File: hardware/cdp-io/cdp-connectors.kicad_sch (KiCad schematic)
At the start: 1 part, among them J1 Conn_01x26_Pin

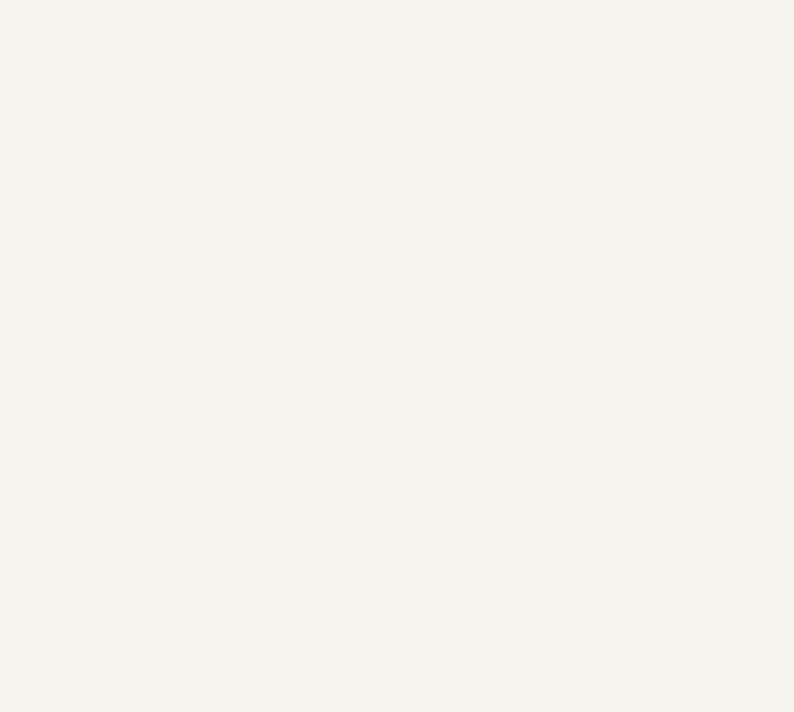
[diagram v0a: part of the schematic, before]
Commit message: A really small progress.
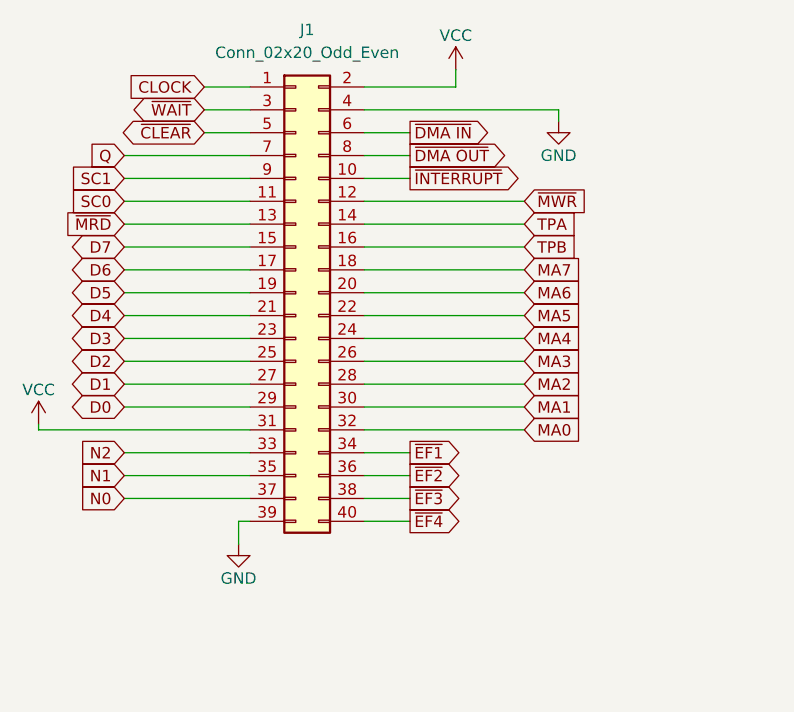
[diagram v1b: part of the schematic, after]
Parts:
- added J1: Conn_02x20_Odd_Even, Connector_IDC:IDC-Header_2x20_P2.54mm_Vertical, symbol Connector_Generic:Conn_02x20_Odd_Even
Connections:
- net GND: now also J1.39 (Pin_39), J1.4 (Pin_4)
- new net CLOCK: J1.1 (Pin_1)
- new net D0: J1.29 (Pin_29)
- new net D1: J1.27 (Pin_27)
- new net D2: J1.25 (Pin_25)
- new net D3: J1.23 (Pin_23)
- new net D4: J1.21 (Pin_21)
- new net D5: J1.19 (Pin_19)
- new net D6: J1.17 (Pin_17)
- new net D7: J1.15 (Pin_15)
- new net MA0: J1.32 (Pin_32)
- new net MA1: J1.30 (Pin_30)
- new net MA2: J1.28 (Pin_28)
- new net MA3: J1.26 (Pin_26)
- new net MA4: J1.24 (Pin_24)
- new net MA5: J1.22 (Pin_22)
- new net MA6: J1.20 (Pin_20)
- new net MA7: J1.18 (Pin_18)
- new net N0: J1.37 (Pin_37)
- new net N1: J1.35 (Pin_35)
- new net N2: J1.33 (Pin_33)
- new net Q: J1.7 (Pin_7)
- new net SC0: J1.11 (Pin_11)
- new net SC1: J1.9 (Pin_9)
- new net TPA: J1.14 (Pin_14)
- new net TPB: J1.16 (Pin_16)
- new net VCC: J1.2 (Pin_2), J1.31 (Pin_31)
- new net ~{CLEAR}: J1.5 (Pin_5)
- new net ~{DMA IN}: J1.6 (Pin_6)
- new net ~{DMA OUT}: J1.8 (Pin_8)
- new net ~{EF1}: J1.34 (Pin_34)
- new net ~{EF2}: J1.36 (Pin_36)
- new net ~{EF3}: J1.38 (Pin_38)
- new net ~{EF4}: J1.40 (Pin_40)
- new net ~{INTERRUPT}: J1.10 (Pin_10)
- new net ~{MRD}: J1.13 (Pin_13)
- new net ~{MWR}: J1.12 (Pin_12)
- new net ~{WAIT}: J1.3 (Pin_3)
